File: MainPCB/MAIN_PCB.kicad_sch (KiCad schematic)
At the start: 11 parts, among them J1 S4B-PH-SM4-TB, J2 S4B-PH-SM4-TB, J3 S4B-PH-SM4-TB, U2 INA226

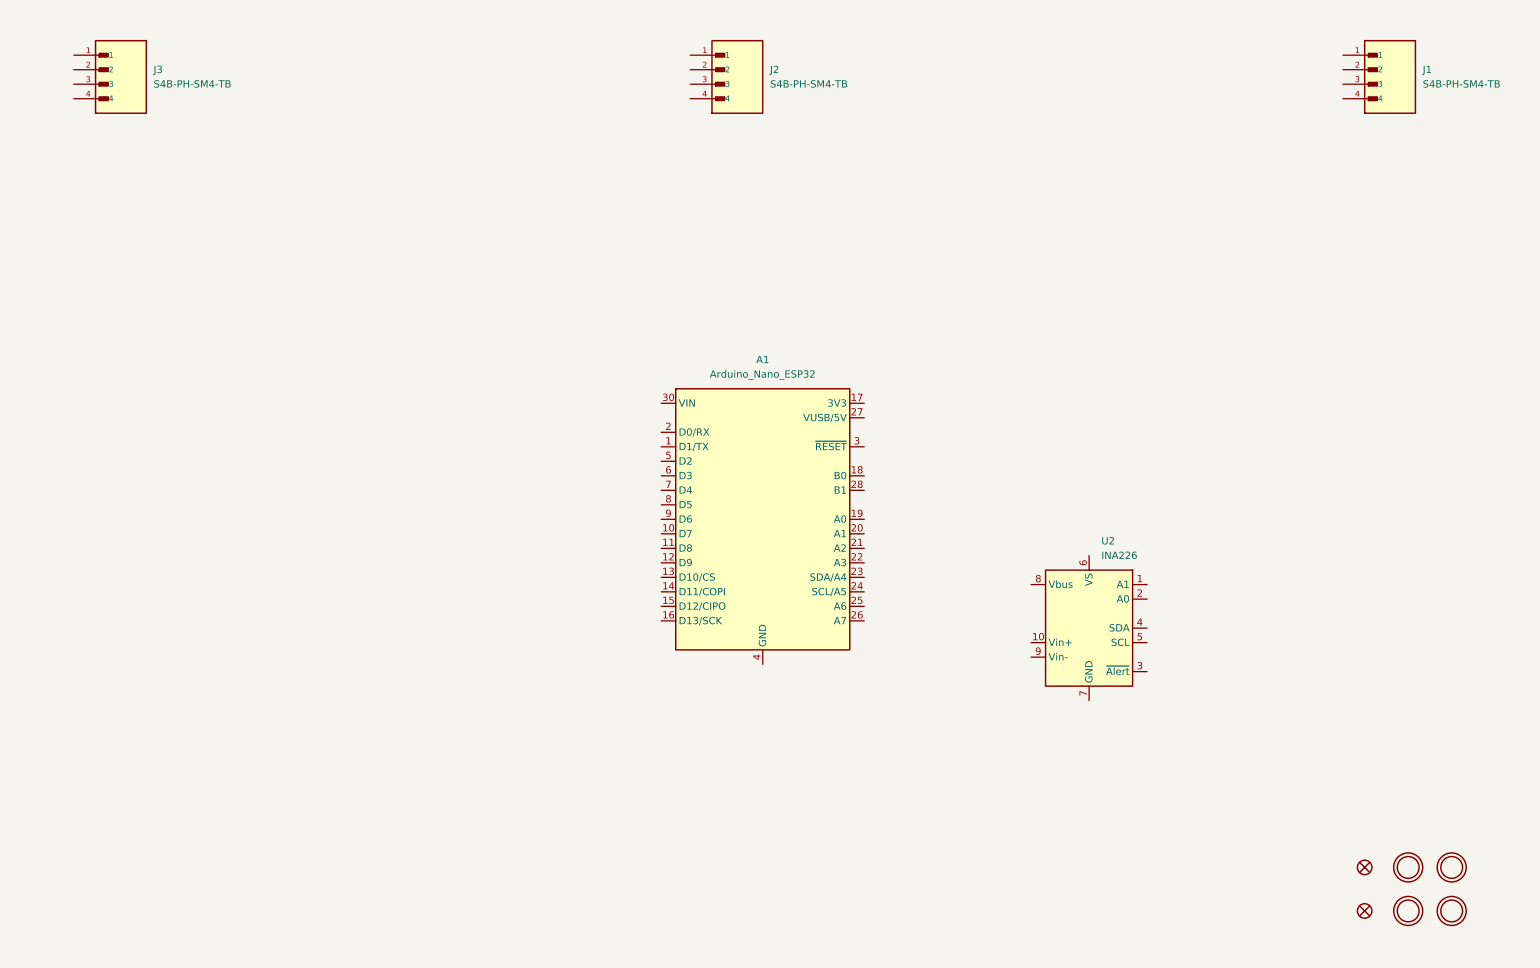
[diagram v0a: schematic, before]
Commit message: a
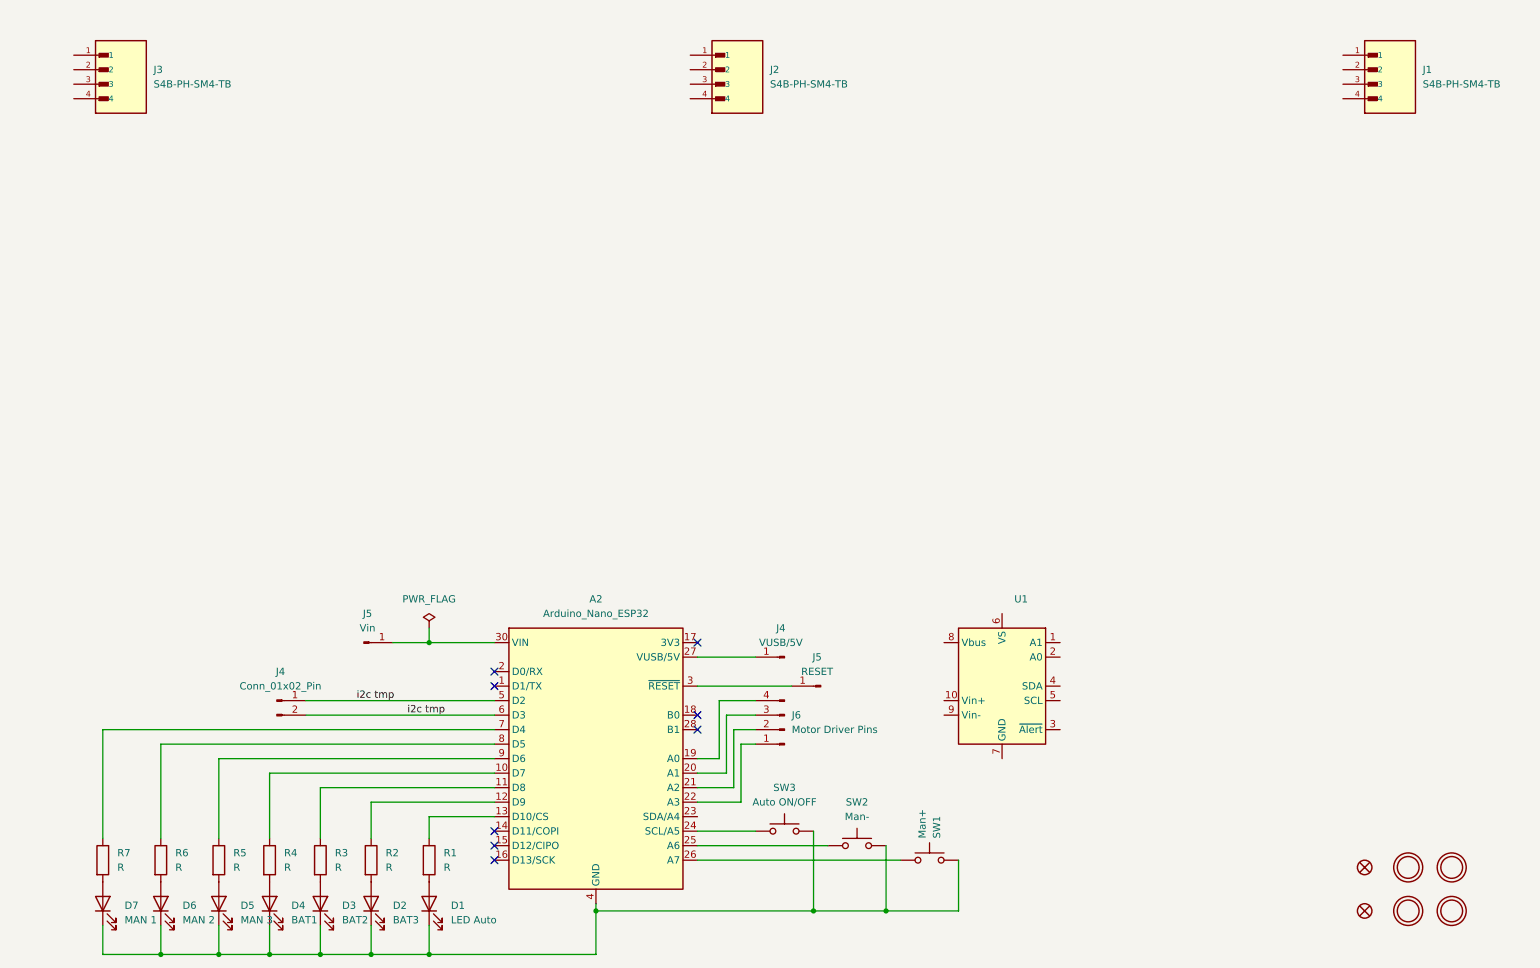
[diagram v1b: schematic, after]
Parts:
- removed A1: Arduino_Nano_ESP32, Module:Arduino_Nano, symbol MCU_Module:Arduino_Nano_ESP32
- removed U2: INA226, Package_SO:VSSOP-10_3x3mm_P0.5mm, symbol Sensor_Energy:INA226
- added A2: Arduino_Nano_ESP32, Module:Arduino_Nano, symbol MCU_Module:Arduino_Nano_ESP32
- added D1: LED Auto, LED_THT:LED_D3.0mm, symbol Device:LED
- added D2: BAT3, LED_THT:LED_D3.0mm, symbol Device:LED
- added D3: BAT2, LED_THT:LED_D3.0mm, symbol Device:LED
- added D4: BAT1, LED_THT:LED_D3.0mm, symbol Device:LED
- added D5: MAN 3, LED_THT:LED_D3.0mm, symbol Device:LED
- added D6: MAN 2, LED_THT:LED_D3.0mm, symbol Device:LED
- added D7: MAN 1, LED_THT:LED_D3.0mm, symbol Device:LED
- added J4: Conn_01x02_Pin, symbol Connector:Conn_01x02_Pin
- added J4: VUSB/5V, Connector_PinHeader_2.54mm:PinHeader_1x01_P2.54mm_Horizontal, symbol Connector:Conn_01x01_Pin
- added J5: RESET, Connector_PinHeader_2.54mm:PinHeader_1x01_P2.54mm_Horizontal, symbol Connector:Conn_01x01_Pin
- added J5: Vin, Connector_PinHeader_2.54mm:PinHeader_1x01_P2.54mm_Horizontal, symbol Connector:Conn_01x01_Pin
- added J6: Motor Driver Pins, symbol Connector:Conn_01x04_Pin
- added R1, R2, R3, R4, R5, R6, R7: R, Resistor_THT:R_Axial_DIN0207_L6.3mm_D2.5mm_P7.62mm_Horizontal, symbol Device:R
- added SW1: Man+, Button_Switch_THT:SW_PUSH_6mm, symbol Switch:SW_Push
- added SW2: Man-, Button_Switch_THT:SW_PUSH_6mm, symbol Switch:SW_Push
- added SW3: Auto ON/OFF, Button_Switch_THT:SW_PUSH_6mm, symbol Switch:SW_Push
- added U1: INA226, Package_SO:VSSOP-10_3x3mm_P0.5mm, symbol Sensor_Energy:INA226
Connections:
- new net: A2.29 (GND), A2.4 (GND), D1.1 (K), D2.1 (K), D3.1 (K), D4.1 (K), D5.1 (K), D6.1 (K), D7.1 (K), SW1.1, SW2.2, SW3.2
- new net: D2.2 (A), R2.2
- new net: A2.26 (A7), SW1.2
- new net: D7.2 (A), R7.2
- new net: D6.2 (A), R6.2
- new net: A2.22 (A3), J6.1 (Pin_1)
- new net: A2.21 (A2), J6.2 (Pin_2)
- new net: A2.20 (A1), J6.3 (Pin_3)
- new net: A2.19 (A0), J6.4 (Pin_4)
- new net: D3.2 (A), R3.2
- new net: A2.12 (D9), R2.1
- new net: A2.9 (D6), R5.1
- new net: D5.2 (A), R5.2
- new net: A2.3 (~{RESET}), J5.1 (Pin_1)
- new net: A2.8 (D5), R6.1
- new net: A2.7 (D4), R7.1
- new net: A2.25 (A6), SW2.1
- new net: A2.27 (VUSB/5V), J4.1 (Pin_1)
- new net: A2.13 (D10/CS), R1.1
- new net: D1.2 (A), R1.2
- new net: A2.24 (SCL/A5), SW3.1
- new net: A2.30 (VIN), J5.1 (Pin_1)
- new net: D4.2 (A), R4.2
- new net: A2.10 (D7), R4.1
- new net: A2.11 (D8), R3.1
- new net i2c tmp: A2.5 (D2), A2.6 (D3), J4.1 (Pin_1), J4.2 (Pin_2)
- no-connect marks 0 -> 8

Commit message: main
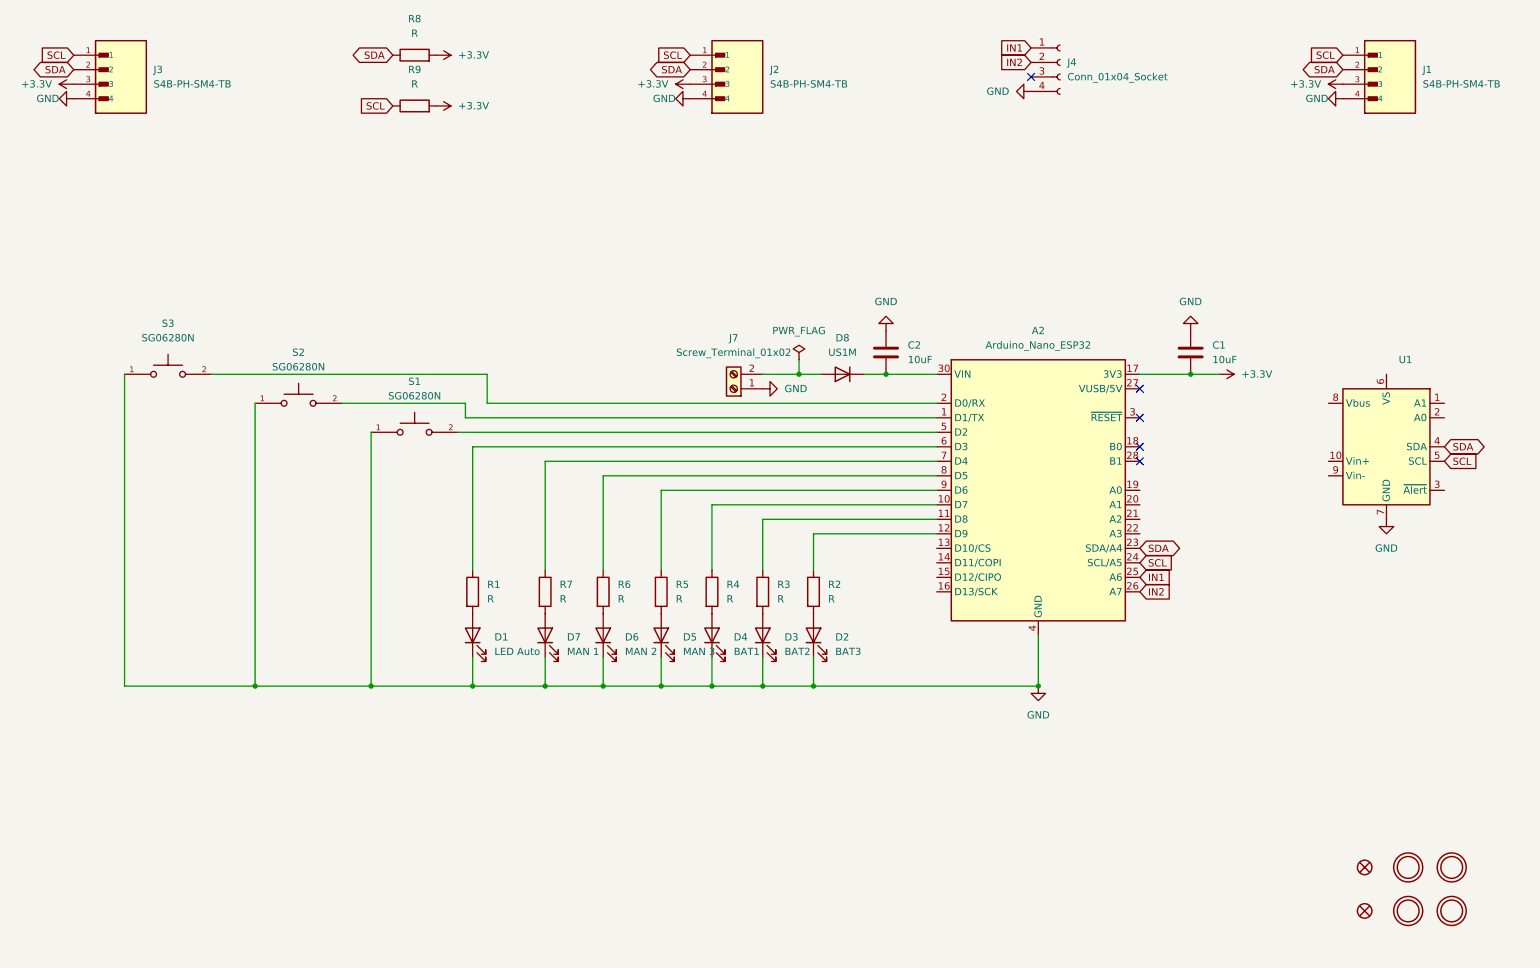
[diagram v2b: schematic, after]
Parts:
- removed J4: Conn_01x02_Pin, symbol Connector:Conn_01x02_Pin
- removed J4: VUSB/5V, Connector_PinHeader_2.54mm:PinHeader_1x01_P2.54mm_Horizontal, symbol Connector:Conn_01x01_Pin
- removed J5: RESET, Connector_PinHeader_2.54mm:PinHeader_1x01_P2.54mm_Horizontal, symbol Connector:Conn_01x01_Pin
- removed J5: Vin, Connector_PinHeader_2.54mm:PinHeader_1x01_P2.54mm_Horizontal, symbol Connector:Conn_01x01_Pin
- removed J6: Motor Driver Pins, symbol Connector:Conn_01x04_Pin
- removed SW1: Man+, Button_Switch_THT:SW_PUSH_6mm, symbol Switch:SW_Push
- removed SW2: Man-, Button_Switch_THT:SW_PUSH_6mm, symbol Switch:SW_Push
- removed SW3: Auto ON/OFF, Button_Switch_THT:SW_PUSH_6mm, symbol Switch:SW_Push
- added C1, C2: 10uF, Capacitor_SMD:C_1206_3216Metric, symbol Device:C
- added D8: US1M, Diode_SMD:D_SMA, symbol Diode:US1M
- added J4: Conn_01x04_Socket, Connector_PinHeader_2.54mm:PinHeader_1x04_P2.54mm_Vertical, symbol Connector:Conn_01x04_Socket
- added J7: Screw_Terminal_01x02, TerminalBlock_4Ucon:TerminalBlock_4Ucon_1x02_P3.50mm_Horizontal, symbol Connector:Screw_Terminal_01x02
- added R8, R9: R, Resistor_THT:R_Axial_DIN0207_L6.3mm_D2.5mm_P7.62mm_Horizontal, symbol Device:R
- added S1, S2, S3: SG06280N, SG06280N:SW_SG06280N, symbol SG06280N:SG06280N
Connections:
- net GND: now reaches A2.29 (GND), A2.4 (GND), D1.1 (K), D2.1 (K), D3.1 (K), D4.1 (K), D5.1 (K), D6.1 (K), D7.1 (K)
- net GND: now also J1.4, J2.4, J3.4, U1.7 (GND), C1.1, C2.1, J4.4 (Pin_4), J7.1 (Pin_1), S1.1, S2.1, S3.1
- net IN2: now reaches A2.26 (A7)
- net IN2: now also J4.2 (Pin_2)
- net SCL: now reaches J3.1
- net SCL: now also A2.24 (SCL/A5), J1.1, J2.1, U1.5 (SCL), R9.1
- net SDA: now reaches J3.2
- net SDA: now also A2.23 (SDA/A4), J1.2, J2.2, U1.4 (SDA), R8.1
- net +3.3V: now reaches J3.3
- net +3.3V: now also A2.17 (3V3), J1.3, J2.3, C1.2, R8.2, R9.2
- net IN1: now reaches A2.25 (A6)
- net IN1: now also J4.1 (Pin_1)
- net at R1.1: now also A2.6 (D3); no longer A2.13 (D10/CS)
- net at A2.30 (VIN): now also C2.2, D8.1 (K)
- net at A2.1 (D1/TX): now also S2.2
- net at A2.2 (D0/RX): now also S3.2
- net i2c tmp: no longer names the net of A2.5 (D2)
- net i2c tmp: now also S1.2; no longer A2.6 (D3)
- new net: D8.2 (A), J7.2 (Pin_2)
- no-connect marks 8 -> 5
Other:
- moved on the sheet: A2, D1, D2, D3, D4, D5, D6, D7, R1, R2, R3, R4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
